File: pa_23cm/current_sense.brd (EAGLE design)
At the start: 101.6 x 101.6 mm, 12 parts, among them IC1 MAX488CSA, IC2 7812T, IC3 7805T, J1 1X2-3.5MM

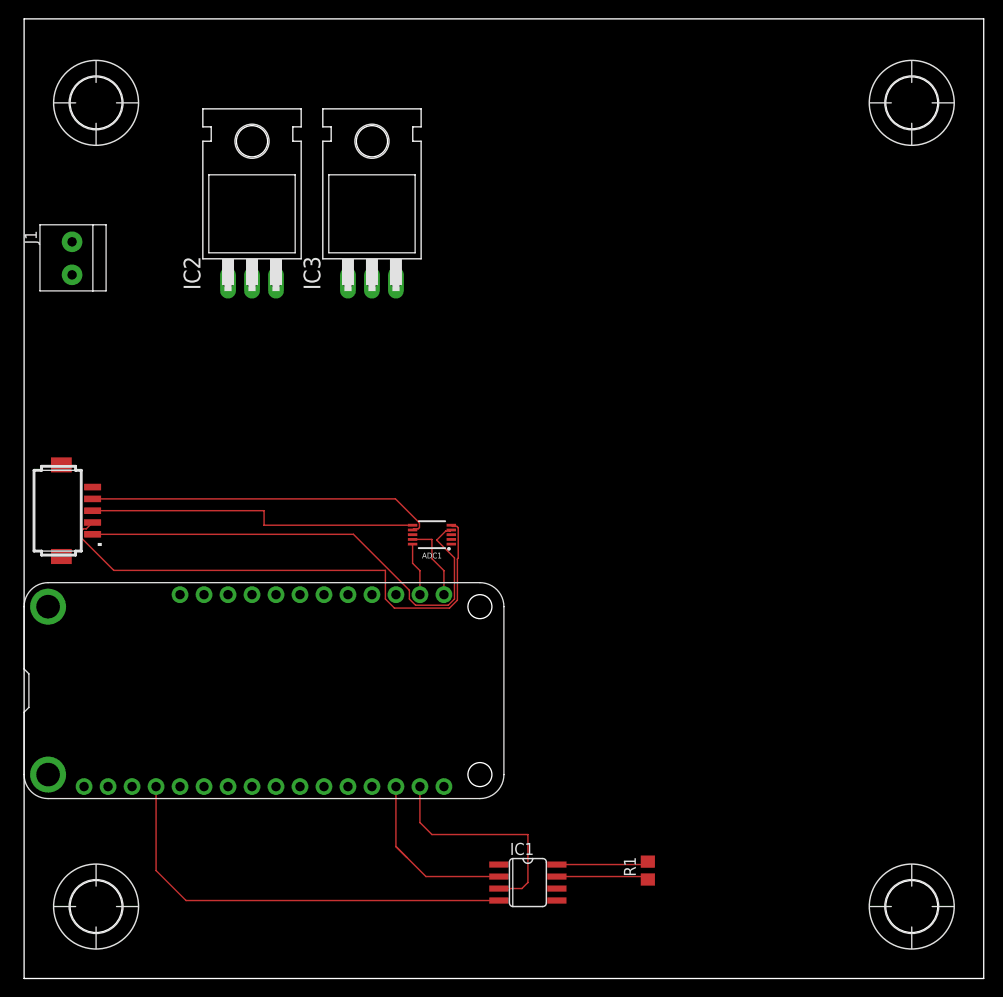
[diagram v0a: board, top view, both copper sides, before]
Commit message: working on current sensor board.  End of day commit.
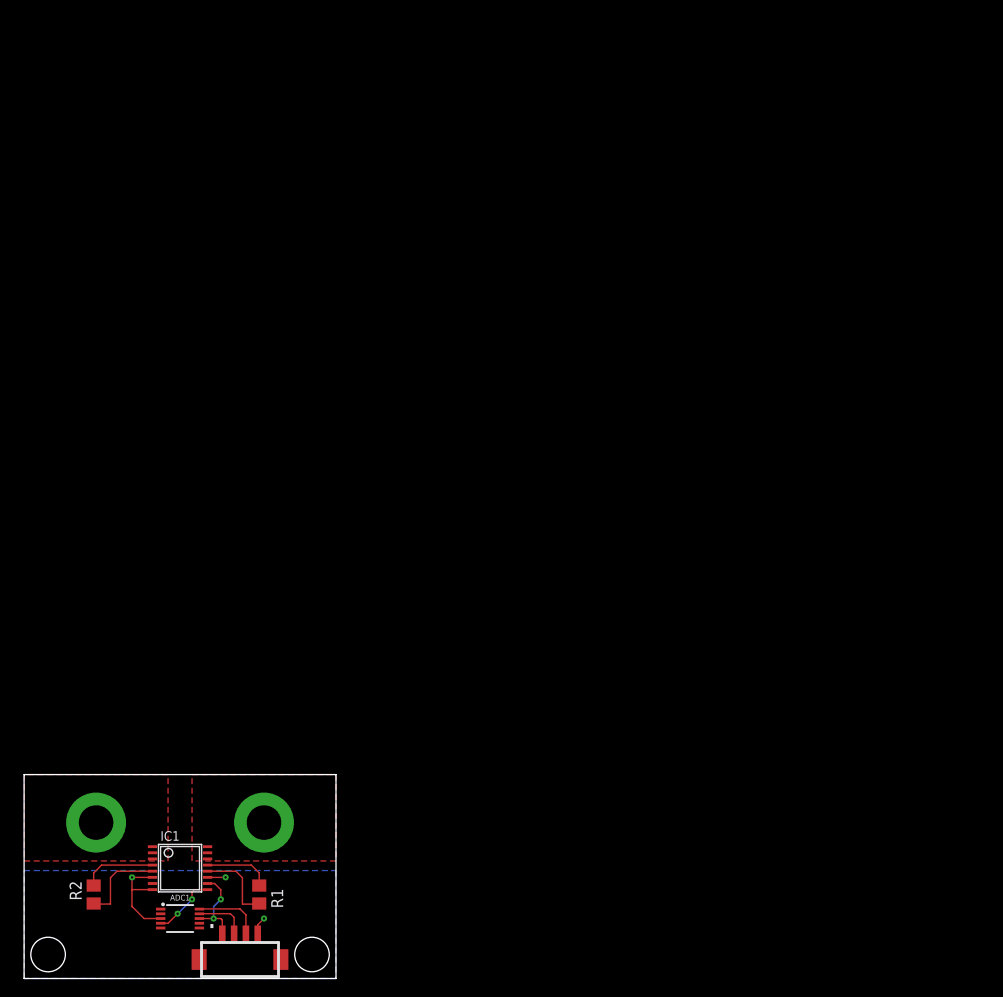
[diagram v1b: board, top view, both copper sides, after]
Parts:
- removed FEATHER_32U4: FEATHERWING_NODIM, adafruit:FEATHERWING_DIM
- removed H1, H2, H3, H4: MOUNT-HOLE5.5, holes:5,5
- removed IC2: 7812T, adafruit:TO220H
- removed IC3: 7805T, adafruit:TO220H
- removed J1: 1X2-3.5MM, adafruit:1X2-3.5MM
- added R2: 0, resistor:R0805
- IC1: value MAX488CSA -> INA250; device maxim:SO08 -> vtgs:TSSOP16
- R1: value 1k -> 0
- U$1: value DF13-5P-1.25H -> DF13-4P-1.25V; device con-hirose-df13:DF13A-5P-1.25H -> con-hirose-df13:DF13C-4P-1.25V
- moved ADC1 48.6 mm to (16.5, 6.35), turned to 270 degrees
- moved U$1 48.6 mm to (22.9, 3.81), turned to 0 degrees
- moved R1 41.2 mm to (24.9, 8.89), turned to 270 degrees
- moved IC1 36.9 mm to (16.5, 11.7)
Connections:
- removed net +12V: IC1.1
- removed net N$2: IC1.7, R1.1
- removed net N$3: ADC1.10, FEATHER_32U4.18
- removed net N$8: ADC1.7, U$1.P$4
- removed net N$9: IC2.1, J1.2
- removed net RXD: FEATHER_32U4.14, IC1.2
- removed net TXD: FEATHER_32U4.15, IC1.3
- new net SCL: ADC1.10, U$1.P$3
- new net SDA: ADC1.9, U$1.P$2
- new net V+: IC1.14, IC1.15, IC1.16
- new net V-: IC1.1, IC1.2, IC1.3
- net +3V3: now also IC1.10, U$1.P$1
- net GND: now also IC1.11, IC1.6, IC1.8, U$1.P$4; no longer FEATHER_32U4.4, IC1.4, J1.1, U$1.P$5
- net N$1: now also ADC1.4, IC1.9; no longer IC1.8, R1.2
- net N$4: now also IC1.4, R2.2; no longer ADC1.9, FEATHER_32U4.17
- net N$5: now also IC1.5, R2.1; no longer ADC1.4, U$1.P$1
- net N$6: now also IC1.13, R1.1; no longer ADC1.5, U$1.P$2
- net N$7: now also IC1.12, R1.2; no longer ADC1.6, U$1.P$3
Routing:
- net N$6: track 55.8 -> 7.15 mm
- net N$5: track 51.3 -> 9.36 mm
- net N$8: track 37.0 -> 0.00 mm
- net GND: track 46.5 -> 14.8 mm, vias 0 -> 3
- net N$7: track 35.4 -> 8.55 mm
- net TXD: track 24.2 -> 0.00 mm
- net RXD: track 20.2 -> 0.00 mm
- net N$2: track 9.76 -> 0.00 mm
- net +3V3: track 0.00 -> 9.01 mm, vias 0 -> 2
- net SCL: track 0.00 -> 7.22 mm
- net N$3: track 5.67 -> 0.00 mm
- net SDA: track 0.00 -> 5.60 mm
- net N$1: track 9.76 -> 6.90 mm, vias 0 -> 2
- net N$4: track 8.43 -> 7.91 mm
- added copper zone on layer 16, net GND
- added copper zone on layer 1, net V+
- added copper zone on layer 1, net V-
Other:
- board size 101.6 x 101.6 mm -> 33 x 21.6 mm
